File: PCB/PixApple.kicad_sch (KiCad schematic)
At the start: 21 parts, among them J3 Conn_01x17, J4 Conn_01x17, J5 Conn_01x05_Pin, J6 Conn_01x02_Pin, SW1 SW_Push, U1 RP2040

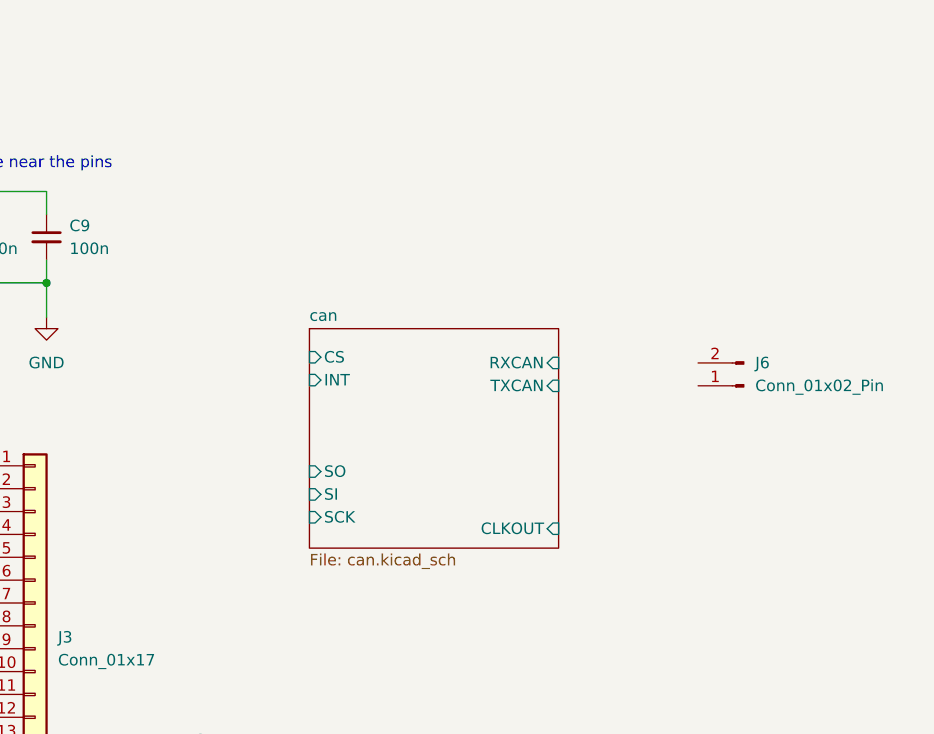
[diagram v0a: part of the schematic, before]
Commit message: CAN bus done?
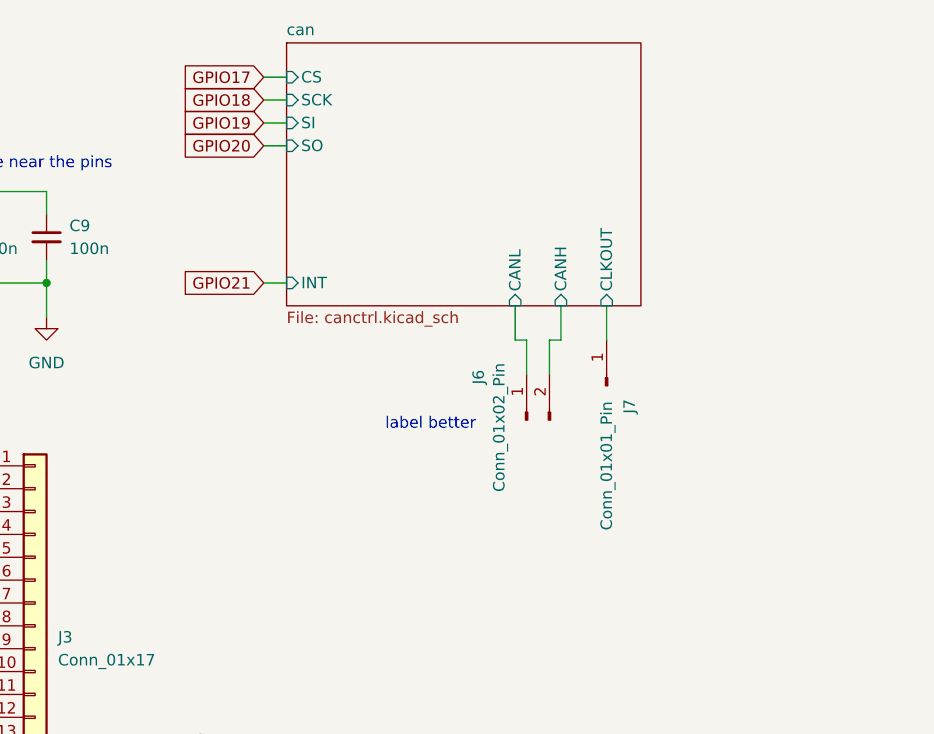
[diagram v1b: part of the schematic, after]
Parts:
- added J7: Conn_01x01_Pin, symbol Connector:Conn_01x01_Pin
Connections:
- net can/CLKOUT: now also J7.1 (Pin_1)
- net can/CANL: now reaches J6.1 (Pin_1)
- net can/CANH: now reaches J6.2 (Pin_2)
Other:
- sheet can: file can.kicad_sch -> canctrl.kicad_sch
- sheet can ports: added CANH, CANL; removed RXCAN, TXCAN
- note added: "label better"
- moved on the sheet: J6

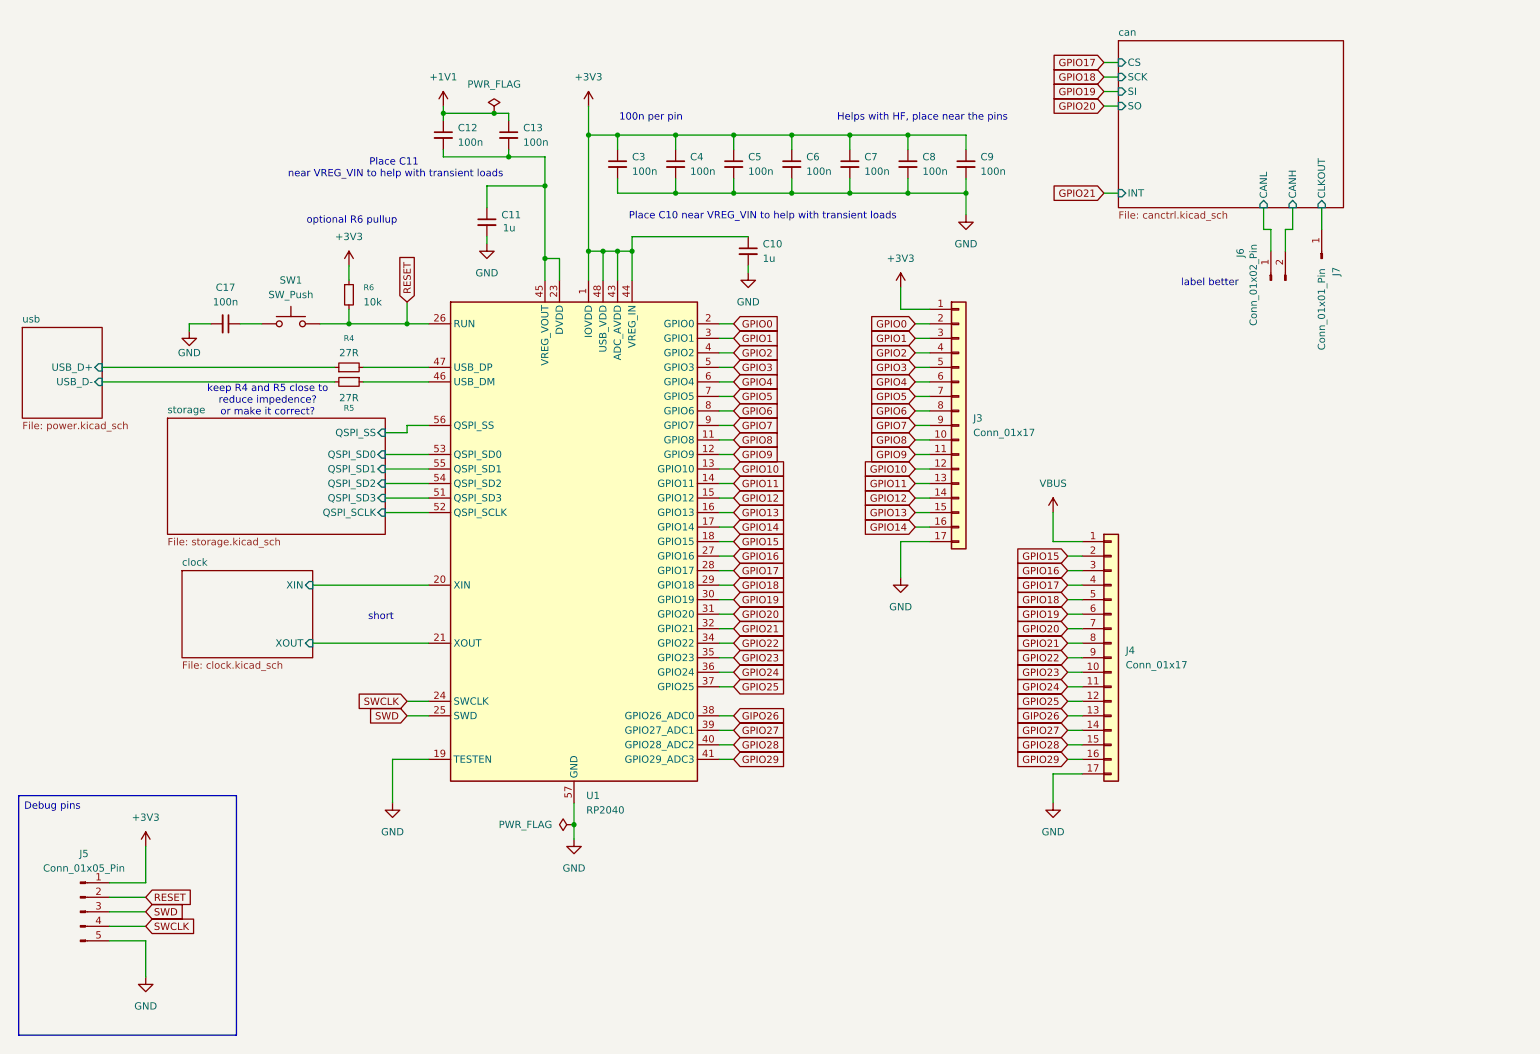
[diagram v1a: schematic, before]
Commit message: Routing PCB
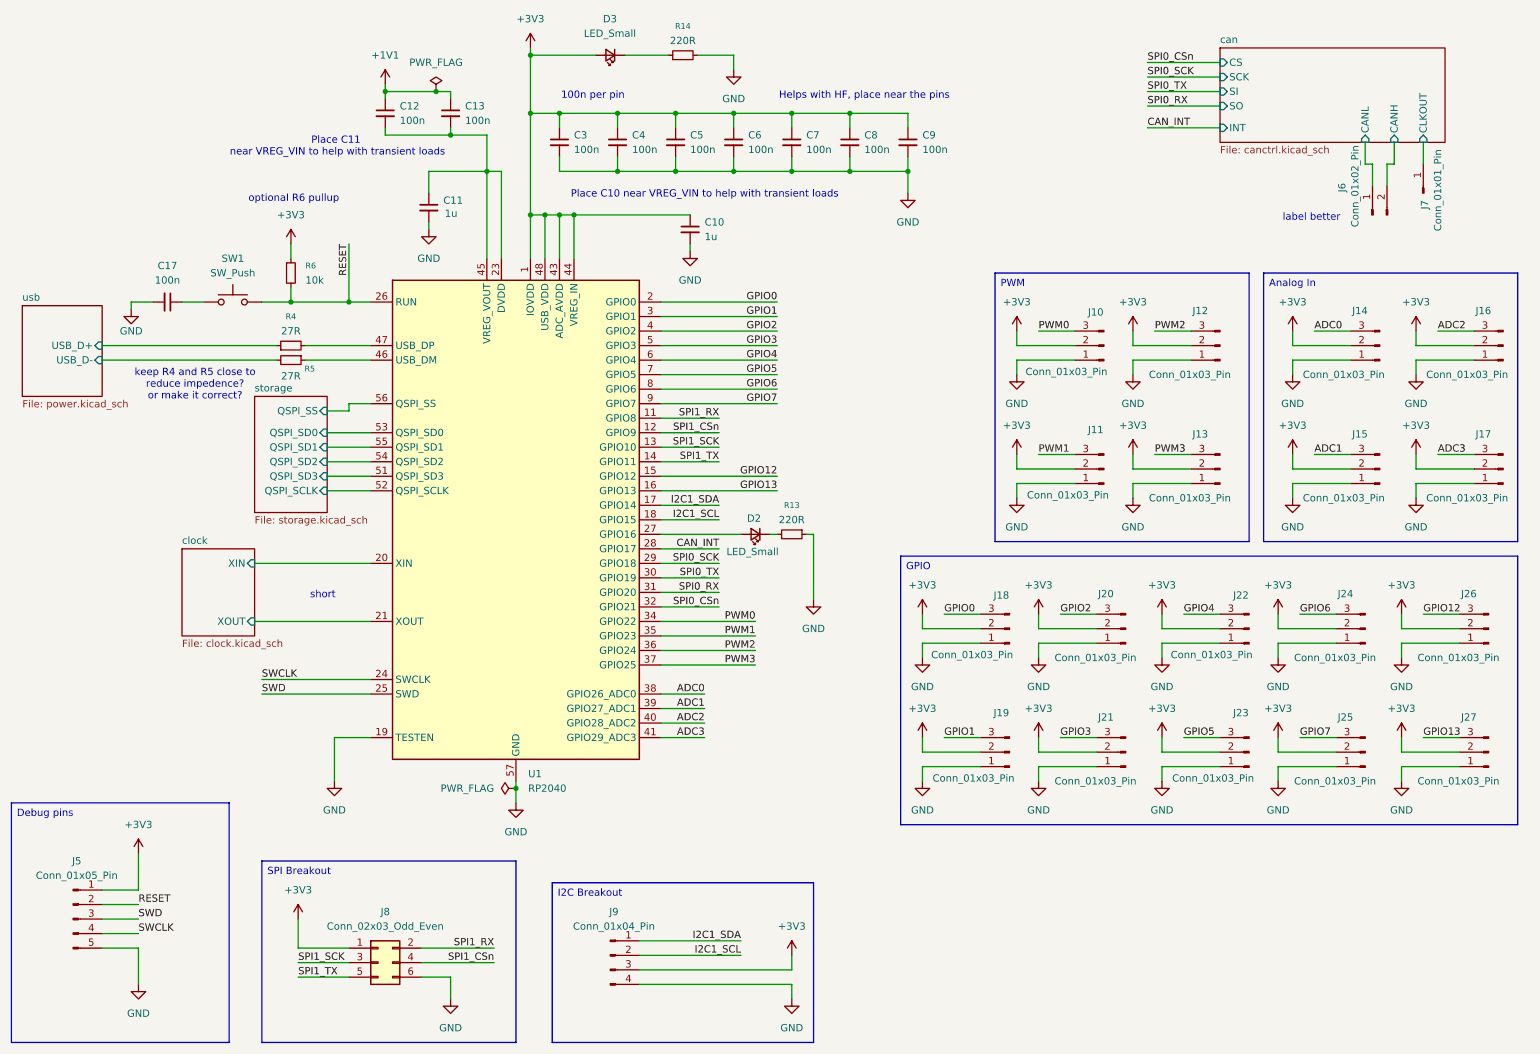
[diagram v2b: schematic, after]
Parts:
- removed J3, J4: Conn_01x17, symbol Connector_Generic:Conn_01x17
- added D2, D3: LED_Small, LED_SMD:LED_0603_1608Metric_Pad1.05x0.95mm_HandSolder, symbol Device:LED_Small
- added J10, J11, J12, J13, J14, J15, J16, J17, J18, J19, J20, J21, J22, J23, J24, J25, J26, J27: Conn_01x03_Pin, Connector_PinHeader_2.54mm:PinHeader_1x03_P2.54mm_Vertical, symbol Connector:Conn_01x03_Pin
- added J8: Conn_02x03_Odd_Even, Connector_PinHeader_2.54mm:PinHeader_2x03_P2.54mm_Vertical, symbol Connector_Generic:Conn_02x03_Odd_Even
- added J9: Conn_01x04_Pin, Connector_PinHeader_2.54mm:PinHeader_1x04_P2.54mm_Vertical, symbol Connector:Conn_01x04_Pin
- added R13, R14: 220R, Resistor_SMD:R_0603_1608Metric_Pad0.98x0.95mm_HandSolder, symbol Device:R_Small
- C10, C11, C12, C13, C17, C3, C4, C5, C6, C7, C8, C9: footprint (none) -> Capacitor_SMD:C_0603_1608Metric_Pad1.08x0.95mm_HandSolder
- J5: footprint (none) -> Connector_PinHeader_2.54mm:PinHeader_1x05_P2.54mm_Vertical
- J6: footprint (none) -> Connector_PinHeader_2.54mm:PinHeader_1x02_P2.54mm_Vertical
- J7: footprint (none) -> TestPoint:TestPoint_Pad_1.0x1.0mm
- R4, R5, R6: footprint (none) -> Resistor_SMD:R_0603_1608Metric_Pad0.98x0.95mm_HandSolder
- SW1: footprint (none) -> Button_Switch_THT:SW_PUSH_6mm_H5mm
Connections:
- net +3V3: now also D3.2 (A), J10.2 (Pin_2), J11.2 (Pin_2), J12.2 (Pin_2), J13.2 (Pin_2), J14.2 (Pin_2), J15.2 (Pin_2), J16.2 (Pin_2), J17.2 (Pin_2), J18.2 (Pin_2), J19.2 (Pin_2), J20.2 (Pin_2), J21.2 (Pin_2), J22.2 (Pin_2), J23.2 (Pin_2), J24.2 (Pin_2), J25.2 (Pin_2), J26.2 (Pin_2), J27.2 (Pin_2), J8.1 (Pin_1), J9.3 (Pin_3)
- net GND: now also J10.1 (Pin_1), J11.1 (Pin_1), J12.1 (Pin_1), J13.1 (Pin_1), J14.1 (Pin_1), J15.1 (Pin_1), J16.1 (Pin_1), J17.1 (Pin_1), J18.1 (Pin_1), J19.1 (Pin_1), J20.1 (Pin_1), J21.1 (Pin_1), J22.1 (Pin_1), J23.1 (Pin_1), J24.1 (Pin_1), J25.1 (Pin_1), J26.1 (Pin_1), J27.1 (Pin_1), J8.6 (Pin_6), J9.4 (Pin_4), R13.1, R14.2
- net GPIO0: now also J18.3 (Pin_3)
- net GPIO1: now also J19.3 (Pin_3)
- net GPIO12: now also J26.3 (Pin_3)
- net GPIO13: now also J27.3 (Pin_3)
- net GPIO2: now also J20.3 (Pin_3)
- net GPIO3: now also J21.3 (Pin_3)
- net GPIO4: now also J22.3 (Pin_3)
- net GPIO5: now also J23.3 (Pin_3)
- net GPIO6: now also J24.3 (Pin_3)
- net GPIO7: now also J25.3 (Pin_3)
- net GIPO26 renamed ADC0
- net ADC0: now also J14.3 (Pin_3)
- net GPIO10 renamed SPI1_SCK
- net SPI1_SCK: now also J8.3 (Pin_3)
- net GPIO11 renamed SPI1_TX
- net SPI1_TX: now also J8.5 (Pin_5)
- net GPIO14 renamed I2C1_SDA
- net I2C1_SDA: now also J9.1 (Pin_1)
- net GPIO15 renamed I2C1_SCL
- net I2C1_SCL: now also J9.2 (Pin_2)
- net GPIO16: no longer names the net of U1.27 (GPIO16)
- net GPIO16: now also D2.2 (A)
- net GPIO17 renamed CAN_INT
- net GPIO18 renamed SPI0_SCK
- net GPIO19 renamed SPI0_TX
- net GPIO20 renamed SPI0_RX
- net GPIO21 renamed SPI0_CSn
- net GPIO22 renamed PWM0
- net PWM0: now also J10.3 (Pin_3)
- net GPIO23 renamed PWM1
- net PWM1: now also J11.3 (Pin_3)
- net GPIO24 renamed PWM2
- net PWM2: now also J12.3 (Pin_3)
- net GPIO25 renamed PWM3
- net PWM3: now also J13.3 (Pin_3)
- net GPIO27 renamed ADC1
- net ADC1: now also J15.3 (Pin_3)
- net GPIO28 renamed ADC2
- net ADC2: now also J16.3 (Pin_3)
- net GPIO29 renamed ADC3
- net ADC3: now also J17.3 (Pin_3)
- net GPIO8 renamed SPI1_RX
- net SPI1_RX: now also J8.2 (Pin_2)
- net GPIO9 renamed SPI1_CSn
- net SPI1_CSn: now also J8.4 (Pin_4)
- new net: D3.1 (K), R14.1
- new net: D2.1 (K), R13.2
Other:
- moved on the sheet: C10, C11, C12, C13, C17, C3, C4, C5, C6, C7, C8, C9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
